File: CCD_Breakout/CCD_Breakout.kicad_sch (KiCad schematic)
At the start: 9 parts, among them U1 ILX511

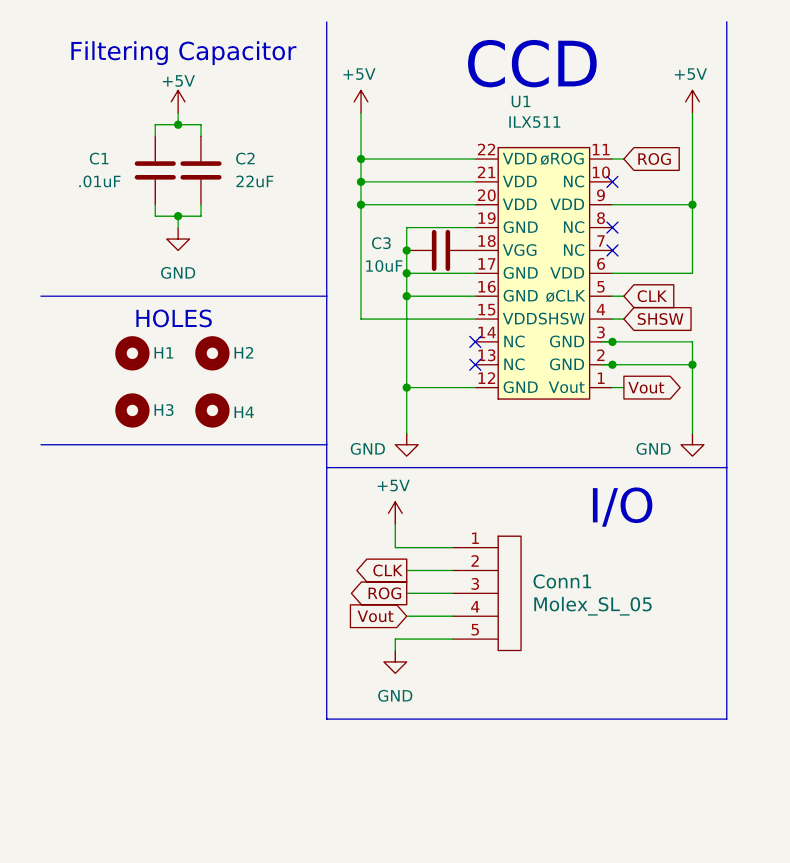
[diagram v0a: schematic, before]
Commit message: updated schematic
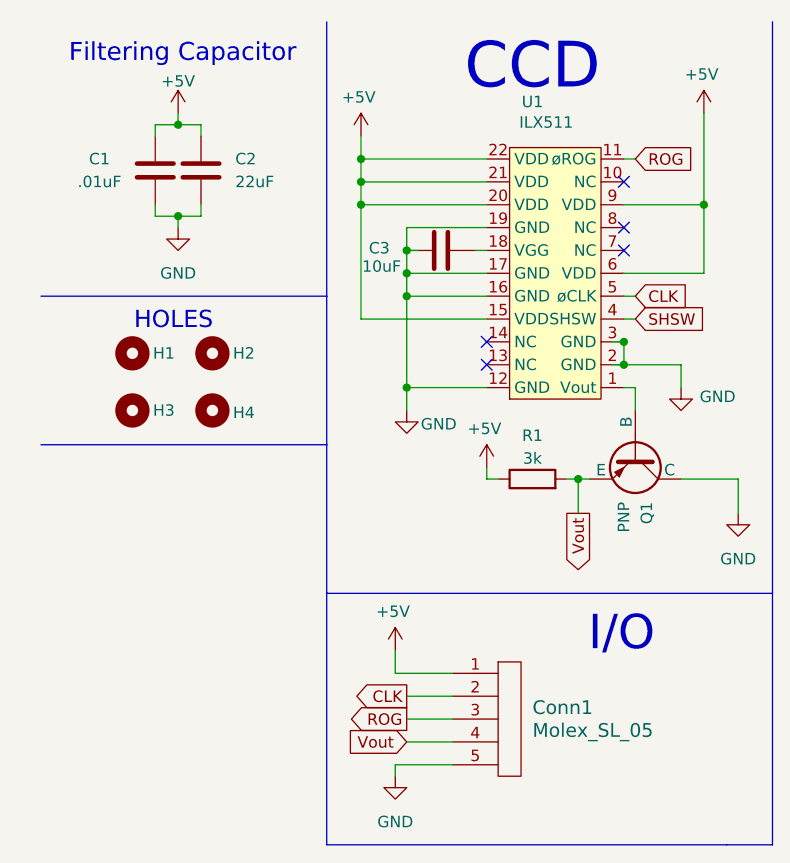
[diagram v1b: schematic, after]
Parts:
- added Q1: PNP, symbol Simulation_SPICE:PNP
- added R1: 3k, symbol Device:R
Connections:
- net +5V: now also R1.1
- net GND: now also Q1.1 (C)
- net Vout: now also Q1.3 (E), R1.2; no longer U1.1 (Vout)
- new net: Q1.2 (B), U1.1 (Vout)
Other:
- moved on the sheet: Conn1, U1
